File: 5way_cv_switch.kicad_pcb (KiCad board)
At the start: 2 copper layers, 29 x 22 mm, 18 parts, among them J1 I/O connector, J2 5-way Switch Connector, U1 HT7550-1, U2 opamp_dbv2

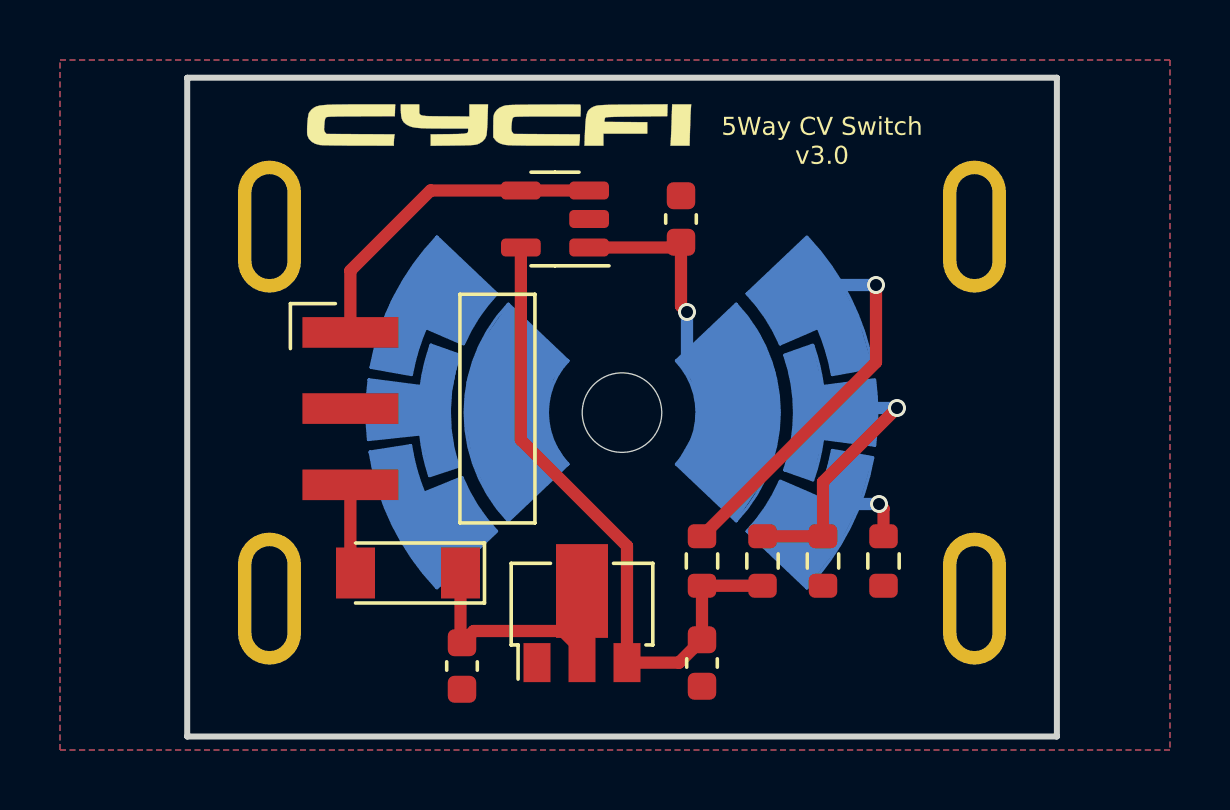
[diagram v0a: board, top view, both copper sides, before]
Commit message: minor updates
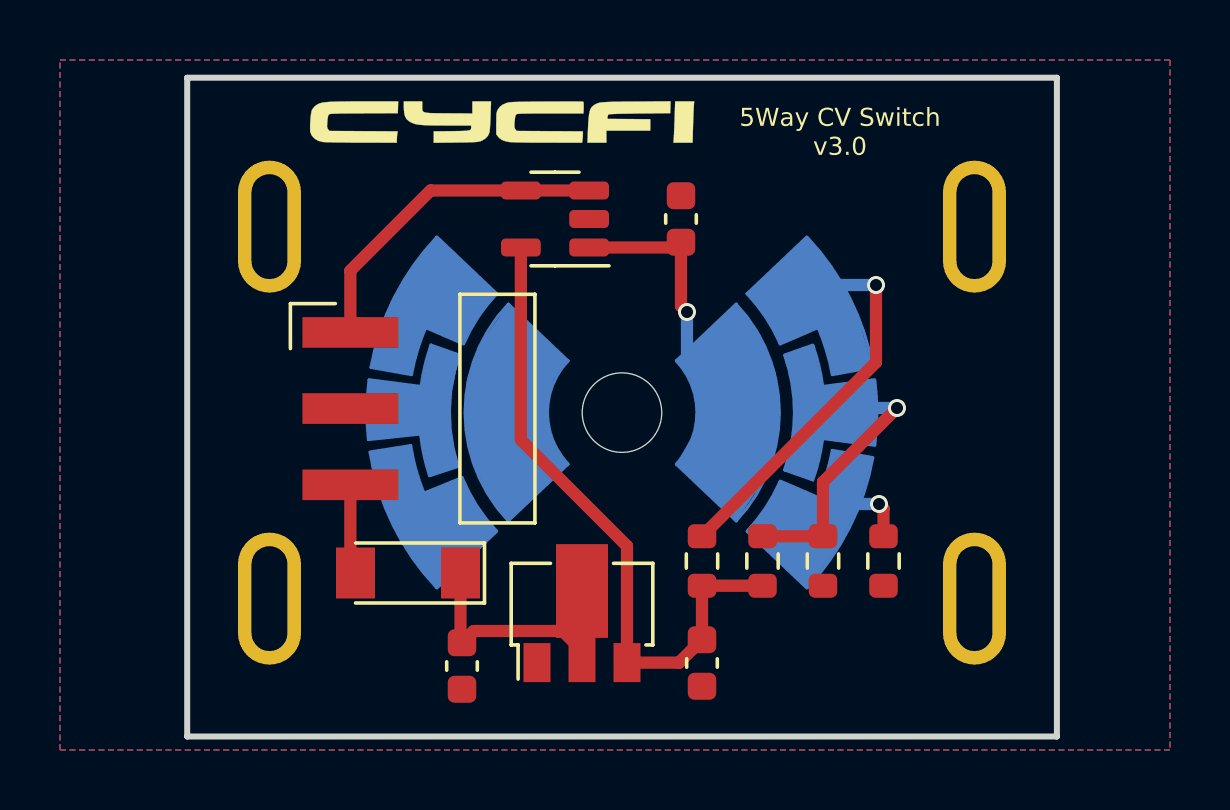
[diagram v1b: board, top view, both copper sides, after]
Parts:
- removed REF**: hole_2.65mm, cycfi_library:hole_2.65mm
- added H5: MountingHole, cycfi_library:hole_2.65mm, F.Cu at (149.7, 49.8)
- moved G*** 0.14 mm to (145.7, 40.1)
